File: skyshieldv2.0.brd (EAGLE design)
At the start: 17.8 x 43.2 mm, 11 parts, among them J1 HEAD15-NOSS, J2 HEAD15-NOSS-1

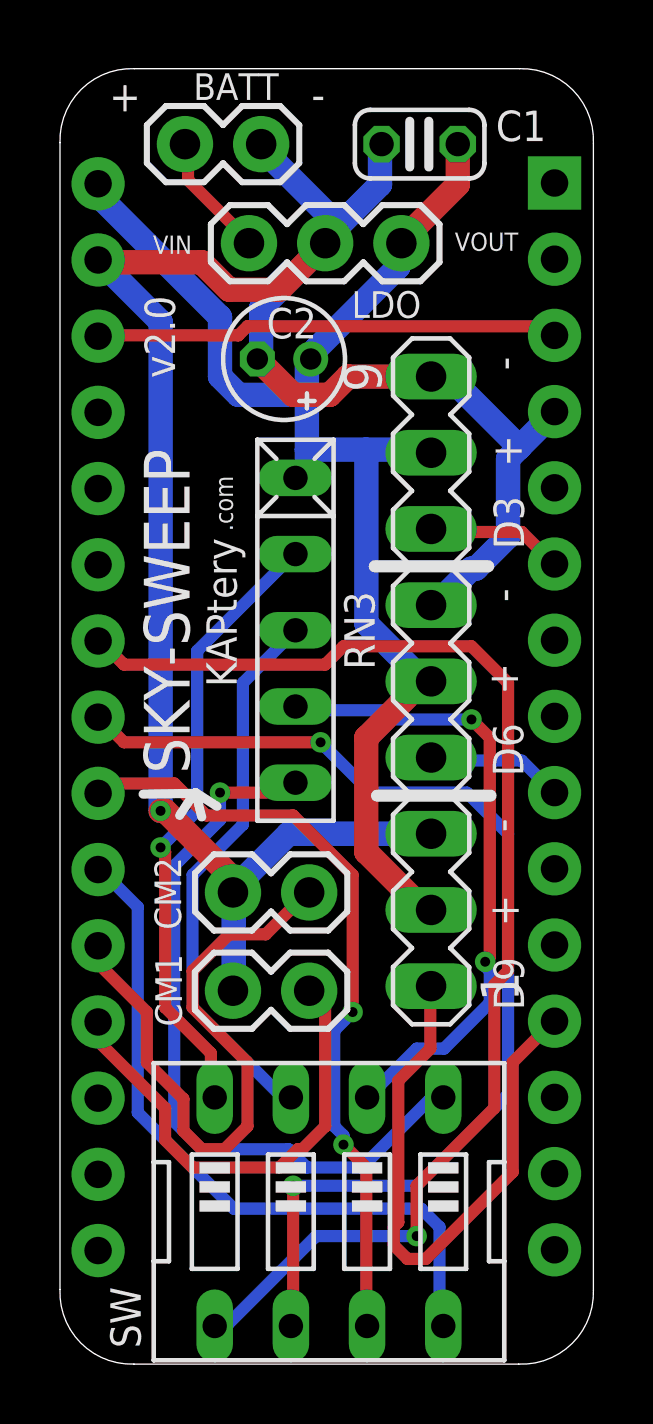
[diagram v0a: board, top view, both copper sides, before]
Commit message: update
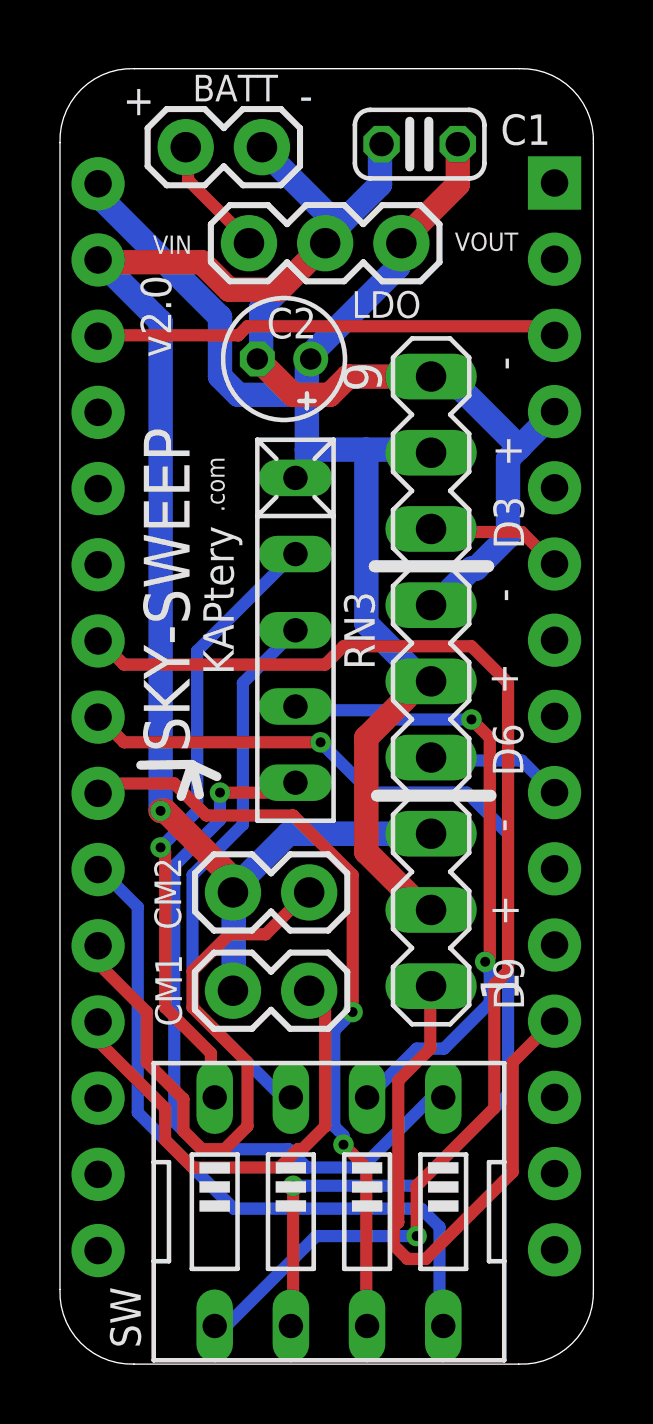
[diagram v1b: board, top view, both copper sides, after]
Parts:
- moved BATT 0.10 mm to (4.19, 40.6)
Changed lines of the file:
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@@
 <wire x1="15.3162" y1="43.18" x2="2.4892" y2="43.18" width="0" layer="20"/>
 <wire x1="0" y1="40.7162" x2="0" y2="2.4892" width="0" layer="20"/>
-<text x="4.318" y="19.685" size="1.524" layer="21" ratio="15" rot="R90">SKY-SWEEP</text>
+<text x="4.318" y="20.3962" size="1.524" layer="21" ratio="15" rot="R90">SKY-SWEEP</text>
 <text x="14.3764" y="30.9626" size="1.016" layer="21" ratio="15" rot="R270">+</text>
 <text x="14.2748" y="33.5788" size="1.016" layer="21" ratio="15" rot="R270">-</text>
@@
 <wire x1="2.4638" y1="0" x2="0" y2="2.4892" width="0" layer="20" curve="-94.264616"/>
 <wire x1="17.78" y1="2.4638" x2="15.2908" y2="0" width="0" layer="20" curve="-94.264616"/>
-<text x="2.6924" y="42.7736" size="1.016" layer="21" ratio="15" rot="R180">+</text>
-<text x="8.382" y="41.8084" size="1.016" layer="21" ratio="15">-</text>
-<text x="4.8768" y="27.5336" size="1.016" layer="21" ratio="15" rot="R270">KAPtery</text>
+<text x="3.1496" y="42.6466" size="1.016" layer="21" ratio="15" rot="R180">+</text>
+<text x="7.9756" y="41.783" size="1.016" layer="21" ratio="15">-</text>
+<text x="4.7752" y="27.94" size="1.016" layer="21" ratio="15" rot="R270">KAPtery</text>
 <text x="14.3002" y="11.7602" size="1.016" layer="22" ratio="15" rot="MR90">publiclab.org/wiki/sky-sweep</text>
 <text x="12.0396" y="35.7632" size="0.889" layer="21" ratio="15" rot="R180">LDO</text>
 <text x="8.5598" y="35.2044" size="1.016" layer="21" ratio="15" rot="R180">C2</text>
-<text x="14.5288" y="40.767" size="1.016" layer="21" ratio="15">C1</text>
-<text x="7.2898" y="43.0276" size="0.889" layer="21" ratio="15" rot="R180">BATT</text>
+<text x="16.3576" y="41.656" size="1.016" layer="21" ratio="15" rot="R180">C1</text>
+<text x="7.2644" y="42.9768" size="0.889" layer="21" ratio="15" rot="R180">BATT</text>
 <text x="13.1572" y="37.1094" size="0.6096" layer="21" font="vector" ratio="15">VOUT</text>
 <text x="3.0988" y="37.0078" size="0.6096" layer="21" font="vector" ratio="15">VIN</text>
-<text x="5.7658" y="27.7622" size="0.6096" layer="21" ratio="15" rot="R90">.com</text>
-<text x="2.8194" y="35.6108" size="1.016" layer="21" ratio="15" rot="R270">v2.0</text>
+<text x="5.4864" y="28.3972" size="0.6096" layer="21" ratio="15" rot="R90">.com</text>
+<text x="2.6924" y="36.2966" size="1.016" layer="21" ratio="15" rot="R270">v2.0</text>
 <text x="5.715" y="4.7752" size="1.4224" layer="22" ratio="15" rot="MR180">KAPtery</text>
 <text x="5.7404" y="3.3274" size="1.016" layer="22" ratio="15" rot="MR0">.com</text>
-<wire x1="4.5212" y1="19.05" x2="5.2324" y2="18.5928" width="0.3048" layer="21"/>
-<wire x1="4.4704" y1="19.0246" x2="2.7686" y2="18.9992" width="0.3048" layer="21"/>
-<wire x1="4.4704" y1="19.0246" x2="3.9878" y2="18.288" width="0.3048" layer="21"/>
-<wire x1="4.5212" y1="19.05" x2="4.7244" y2="18.2372" width="0.3048" layer="21"/>
+<wire x1="4.4196" y1="19.9644" x2="5.2324" y2="19.5834" width="0.3048" layer="21"/>
+<wire x1="4.3942" y1="19.9898" x2="2.6924" y2="19.9644" width="0.3048" layer="21"/>
+<wire x1="4.3942" y1="19.9898" x2="4.0386" y2="18.923" width="0.3048" layer="21"/>
+<wire x1="4.4196" y1="19.9644" x2="4.6482" y2="18.9738" width="0.3048" layer="21"/>
 </plain>
 <attributes>
@@
 <attribute name="VALUE" x="15.2908" y="22.7584" size="1.27" layer="27" ratio="10" rot="R90"/>
 </element>
-<element name="BATT" library="SparkFun-Connectors" package="1X02" value="" x="4.1656" y="40.6654" smashed="yes">
-<attribute name="VALUE" x="2.8956" y="37.4904" size="1.27" layer="27"/>
+<element name="BATT" library="SparkFun-Connectors" package="1X02" value="" x="4.191" y="40.5638" smashed="yes">
+<attribute name="VALUE" x="2.921" y="37.3888" size="1.27" layer="27"/>
 </element>
 <element name="CHDKA" library="SparkFun-Connectors" package="1X02" value="" x="5.7658" y="12.446" smashed="yes">
@@
 <wire x1="8.8392" y1="37.338" x2="8.8392" y2="37.3634" width="0.8128" layer="1"/>
 <wire x1="9.144" y1="38.1" x2="6.7056" y2="40.5384" width="0.8128" layer="16"/>
-<wire x1="6.7056" y1="40.5384" x2="6.7056" y2="40.6654" width="0.8128" layer="16"/>
+<wire x1="6.7056" y1="40.5384" x2="6.731" y2="40.5638" width="0.8128" layer="16"/>
 <wire x1="9.144" y1="38.1" x2="8.8392" y2="37.3634" width="0.8128" layer="16"/>
 <wire x1="9.6012" y1="32.9184" x2="12.3698" y2="32.9184" width="0.8128" layer="1"/>
@@
 <wire x1="4.2672" y1="39.4716" x2="4.2672" y2="40.5384" width="0.4064" layer="1"/>
 <wire x1="6.2484" y1="37.4904" x2="4.2672" y2="39.4716" width="0.4064" layer="1"/>
-<wire x1="4.2672" y1="40.5384" x2="4.1656" y2="40.6654" width="0.4064" layer="1"/>
+<wire x1="4.2672" y1="40.5384" x2="4.191" y2="40.5638" width="0.4064" layer="1"/>
 <wire x1="6.2484" y1="37.4904" x2="6.2992" y2="37.3634" width="0.4064" layer="1"/>
 </signal>
